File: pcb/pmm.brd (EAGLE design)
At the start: 30 x 30 mm, 25 parts, among them IC3 STM32F042F4, SW3 324_SW, SW4 324_SW, U2 USBC_16P, U4 XC6206_DEV

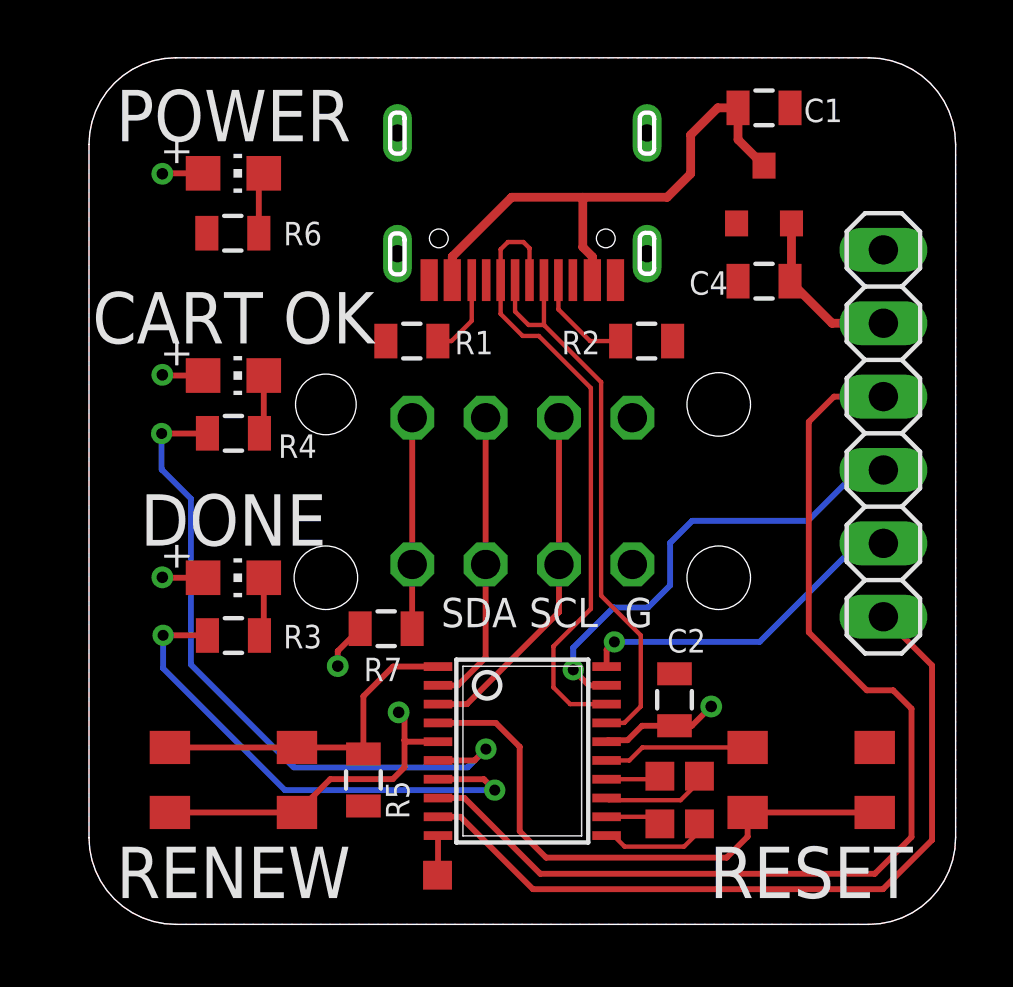
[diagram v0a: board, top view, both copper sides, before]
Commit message: minor adjustments on PCB
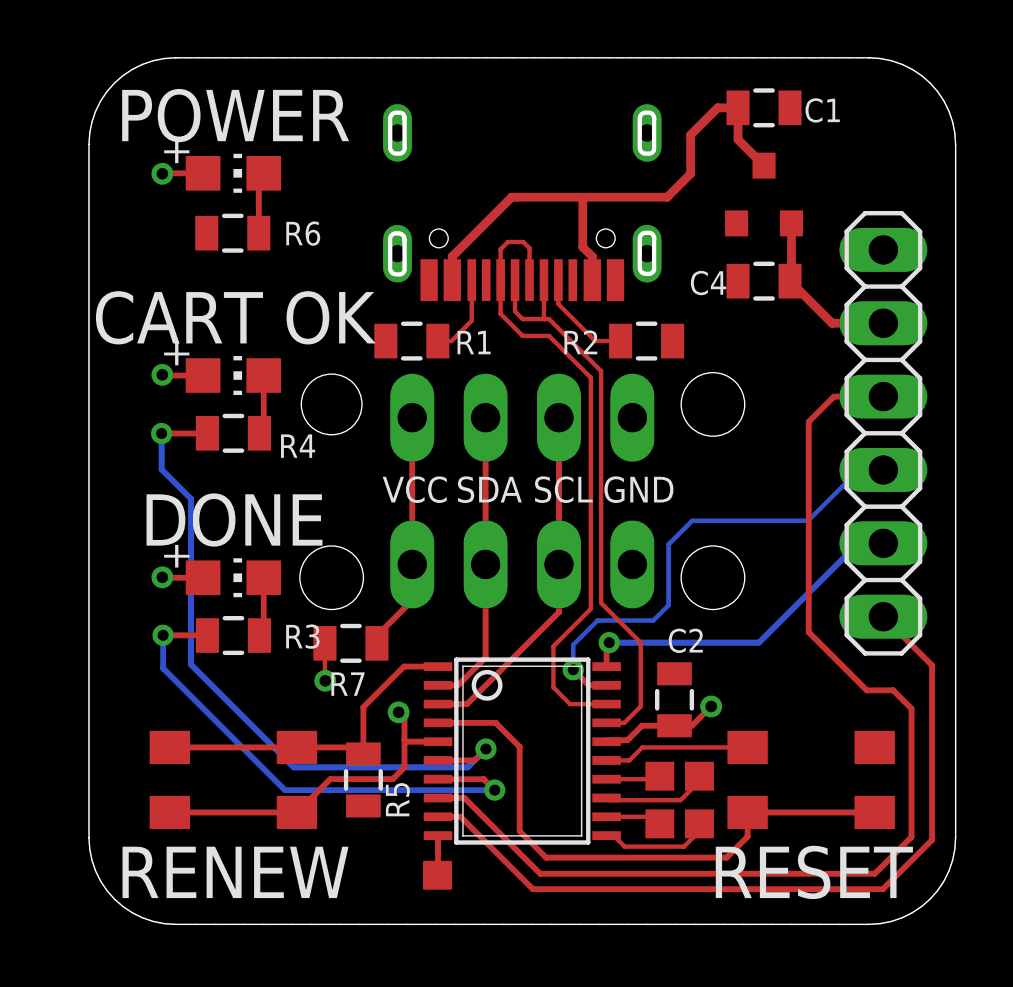
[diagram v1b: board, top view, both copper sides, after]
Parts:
- moved R7 1.32 mm to (9.07, 9.73)
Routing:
- net N$10: track 7.31 -> 8.32 mm
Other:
- board text added: "GND"
- board text added: "VCC"
